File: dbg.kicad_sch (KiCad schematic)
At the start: 30 parts, among them J4 USB_C_Receptacle_USB2.0_16P, J5 Conn_02x05_Odd_Even, SW1 SKRPANE010, U4 USBLC6-2SC6, U5 AP2112K-3.3, U6 STM32F103C8Tx, Y2 8 MHz

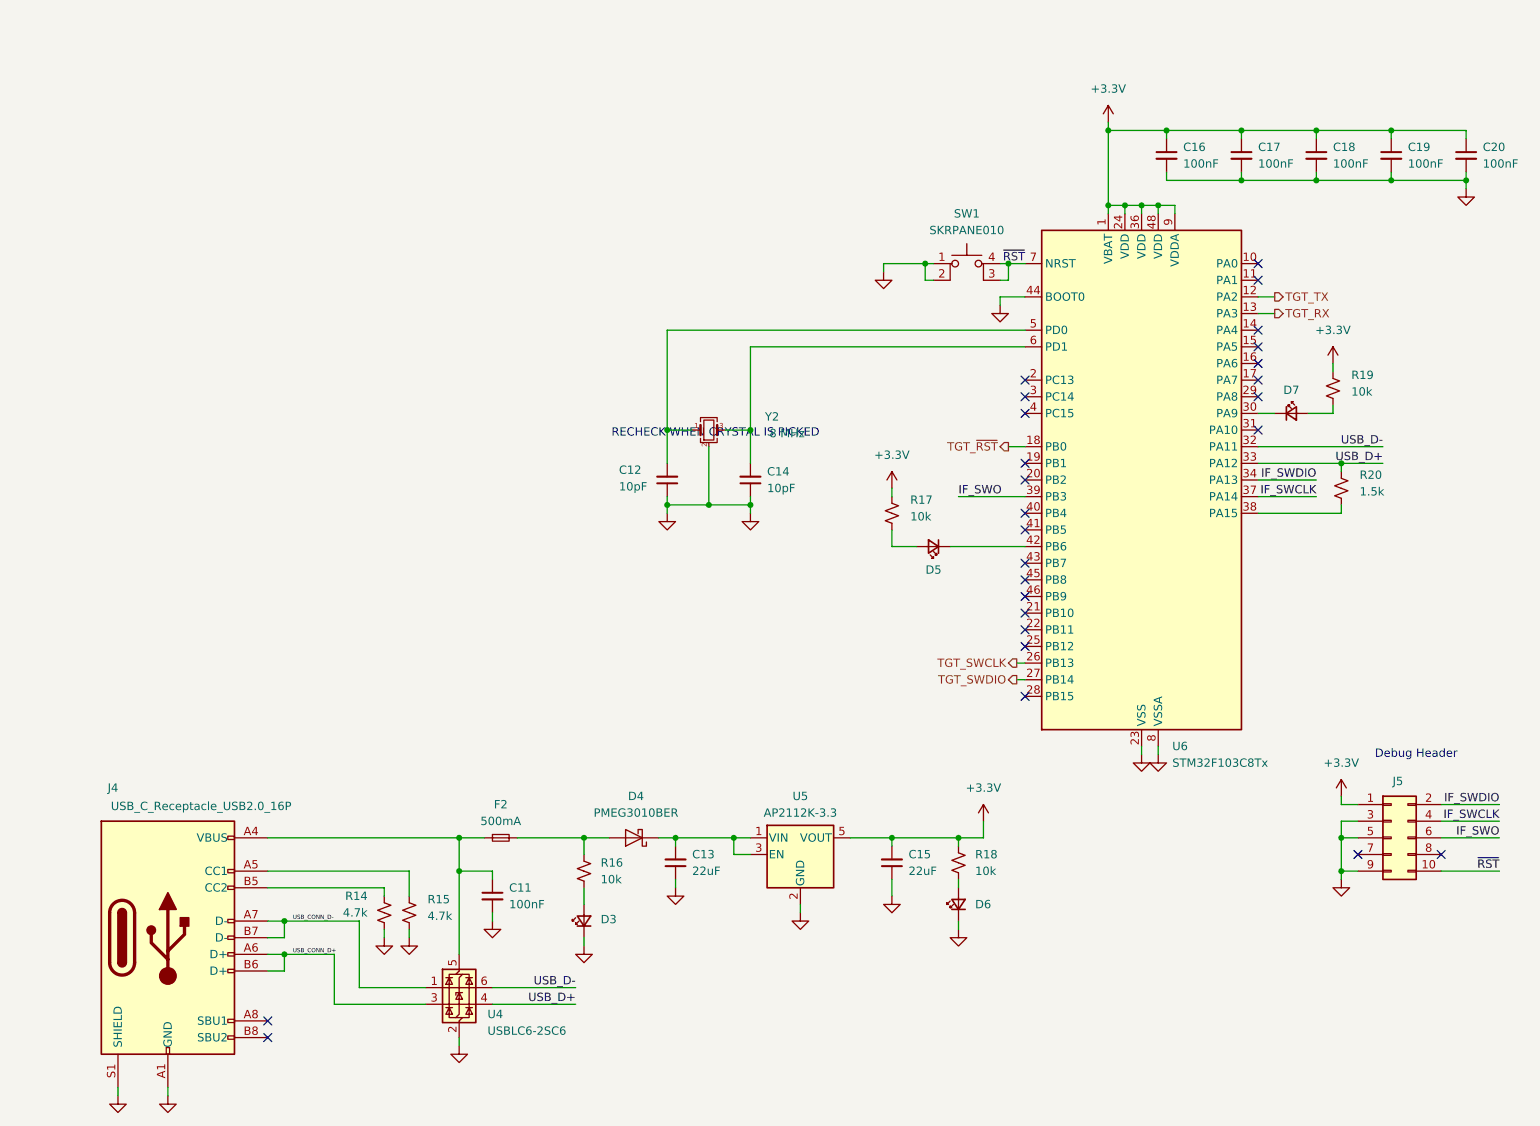
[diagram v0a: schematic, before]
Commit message: ???
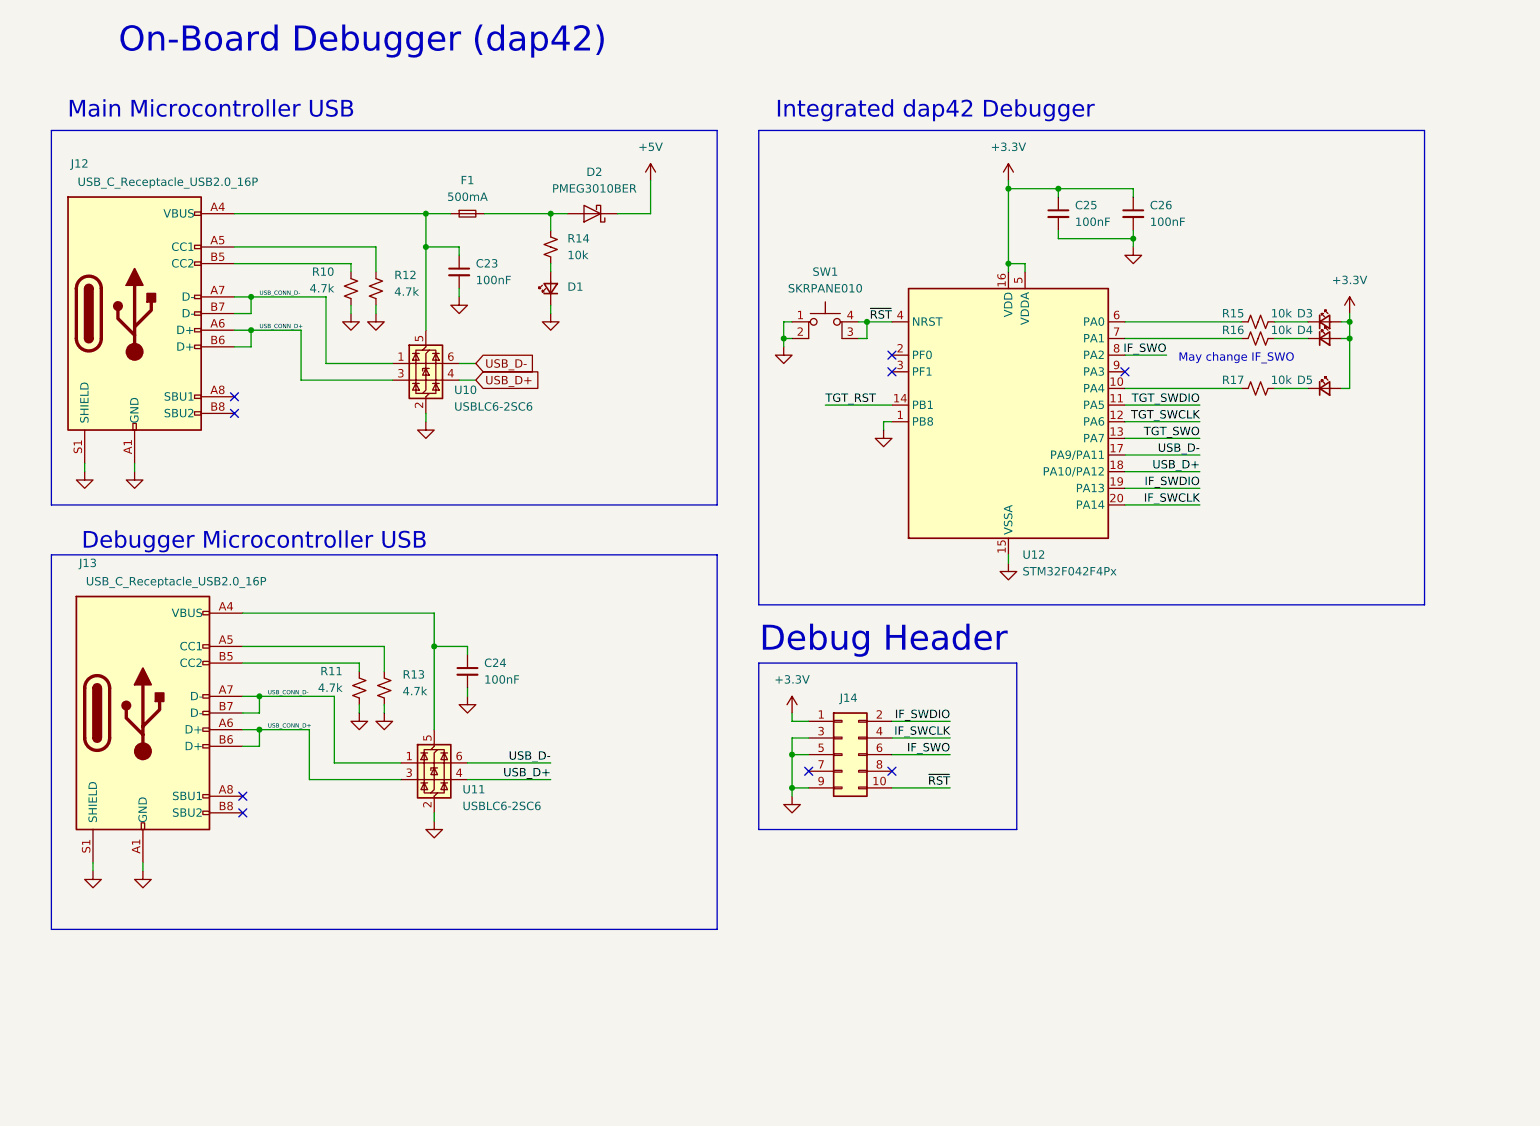
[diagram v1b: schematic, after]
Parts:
- removed C12, C14: 10pF, APRLPrints:C_0603, symbol Device:C_Small
- removed C13, C15: 22uF, APRLPrints:C_0805, symbol Device:C_Small
- removed C16, C17, C18: 100nF, APRLPrints:C_0603, symbol Device:C_Small
- removed D4: PMEG3010BER, Diode_SMD:Nexperia_CFP3_SOD-123W, symbol Diode:PMEG3010BER
- removed D6, D7: LED_Small, APRLPrints:LED_0603, symbol Device:LED_Small
- removed F2: 500mA, Fuse:Fuse_0805_2012Metric, symbol Device:Fuse_Small
- removed R18, R19: 10k, APRLPrints:R_0603, symbol Device:R_Small_US
- removed R20: 1.5k, APRLPrints:R_0603, symbol Device:R_Small_US
- removed U5: AP2112K-3.3, Package_TO_SOT_SMD:SOT-23-5, symbol Regulator_Linear:AP2112K-3.3
- removed U6: STM32F103C8Tx, Package_QFP:LQFP-48_7x7mm_P0.5mm, symbol MCU_ST_STM32F1:STM32F103C8Tx
- removed Y2: 8 MHz, APRLPrints:3225-4P-L, symbol Device:Crystal_GND24_Small
- added C23: 100nF, APRLPrints:C_0603, symbol Device:C_Small
- added D1, D4: LED_Small, APRLPrints:LED_0603, symbol Device:LED_Small
- added D2: PMEG3010BER, Diode_SMD:Nexperia_CFP3_SOD-123W, symbol Diode:PMEG3010BER
- added F1: 500mA, Fuse:Fuse_0805_2012Metric, symbol Device:Fuse_Small
- added J12: USB_C_Receptacle_USB2.0_16P, Connector_USB:USB_C_Receptacle_HRO_TYPE-C-31-M-12, symbol Connector:USB_C_Receptacle_USB2.0_16P
- added R10, R12: 4.7k, APRLPrints:R_0603, symbol Device:R_Small_US
- added R14, R15: 10k, APRLPrints:R_0603, symbol Device:R_Small_US
- added U10: USBLC6-2SC6, Package_TO_SOT_SMD:SOT-23-6, symbol Power_Protection:USBLC6-2SC6
- added U12: STM32F042F4Px, Package_SO:TSSOP-20_4.4x6.5mm_P0.65mm, symbol MCU_ST_STM32F0:STM32F042F4Px
- renumbered C11 to C24, C19 to C25, C20 to C26, J4 to J13, J5 to J14, R14 to R11, R15 to R13, U4 to U11
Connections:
- net +3.3V: now also D3.2 (A), D5.2 (A), D4.2 (A), U12.16 (VDD), U12.5 (VDDA); no longer R17.1
- net GND: now also C23.2, D1.1 (K), J12.A1 (GND), J12.A12 (GND), J12.B1 (GND), J12.B12 (GND), J12.S1 (SHIELD), R10.1, R12.2, U10.2 (GND), U12.1 (PB8), U12.15 (VSSA); no longer D3.1 (K)
- net IF_SWCLK: now also U12.20 (PA14)
- net IF_SWDIO: now also U12.19 (PA13)
- net IF_SWO: now also U12.8 (PA2)
- net TGT_SWCLK: now also U12.12 (PA6)
- net TGT_SWDIO: now also U12.11 (PA5)
- net USB_CONN_D+: now also J12.A6 (D+), J12.B6 (D+), U10.3 (I/O2)
- net USB_CONN_D-: now also J12.A7 (D-), J12.B7 (D-), U10.1 (I/O1)
- net USB_D+: now also U10.4 (I/O2), U12.18 (PA10/PA12)
- net USB_D-: now also U10.6 (I/O1), U12.17 (PA9/PA11)
- net ~{RST}: now also U12.4 (NRST)
- net at R17.2: now also U12.10 (PA4); no longer D5.2 (A)
- net at R16.1: now also D4.1 (K)
- net at R16.2: now also U12.7 (PA1); no longer D3.2 (A)
- net at D5.1 (K): now also R17.1
- new net: J12.A5 (CC1), R12.1
- new net: D3.1 (K), R15.1
- new net: C23.1, F1.1, J12.A4 (VBUS), J12.A9 (VBUS), J12.B4 (VBUS), J12.B9 (VBUS), U10.5 (VBUS)
- new net: J12.B5 (CC2), R10.2
- new net: R15.2, U12.6 (PA0)
- new net: D2.2 (A), F1.2, R14.1
- new net: D1.2 (A), R14.2
- new net +5V: D2.1 (K)
- new net TGT_RST: U12.14 (PB1)
- new net TGT_SWO: U12.13 (PA7)
- no-connect marks 26 -> 9
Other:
- note added: "Debugger Microcontroller USB"
- note added: "Integrated dap42 Debugger"
- note added: "Main Microcontroller USB"
- note added: "May change IF_SWO"
- note added: "On-Board Debugger (dap42)"
- note removed: "RECHECK WHEN CRYSTAL IS PICKED"
- moved on the sheet: C24, C25, C26, J13, J14, R11, R13, U11
